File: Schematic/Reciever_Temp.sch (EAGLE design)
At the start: 5 parts, among them IC1 ATMEGA328P, IC2 LTC485N, IC3 78L05Z, IC4 LM50

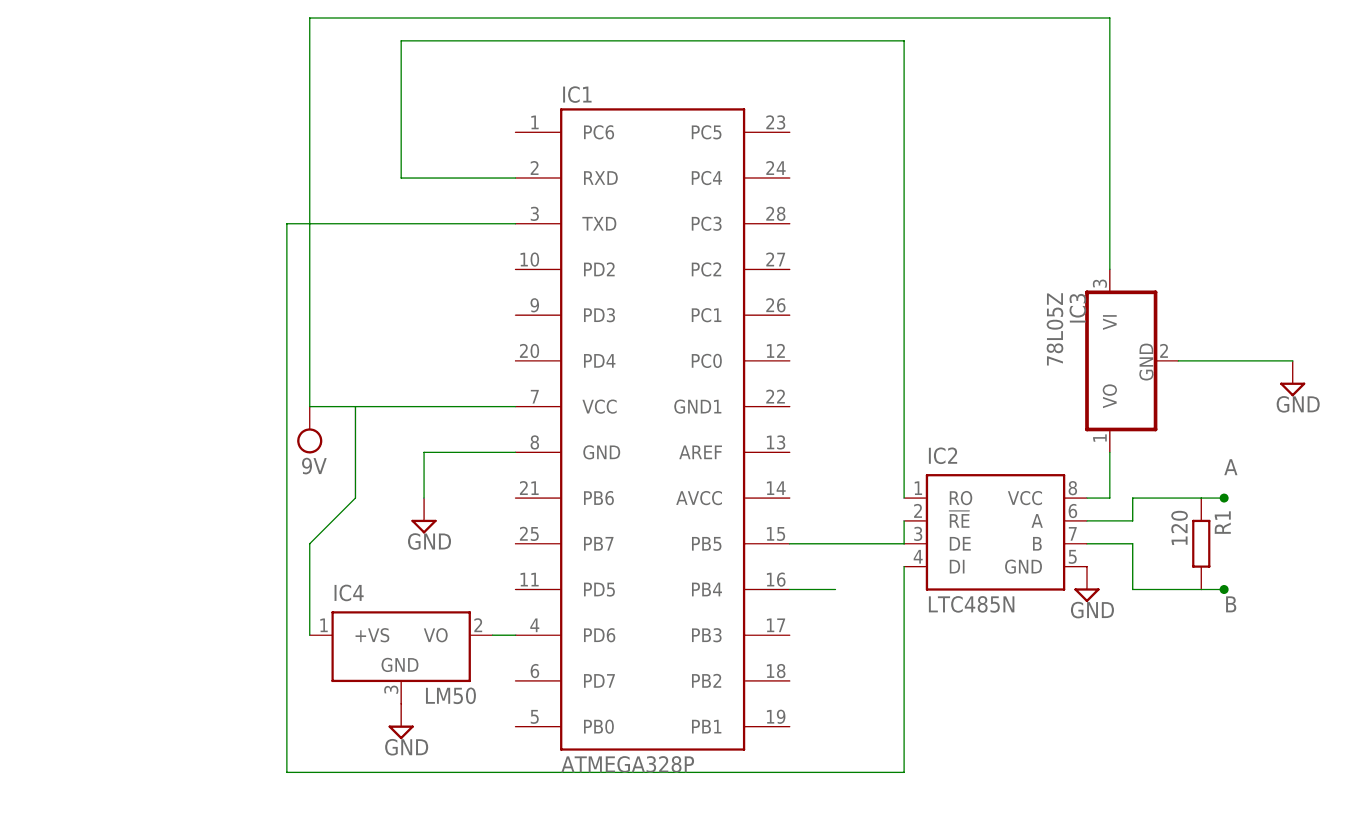
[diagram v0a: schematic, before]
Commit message: Gør klar til eksamen
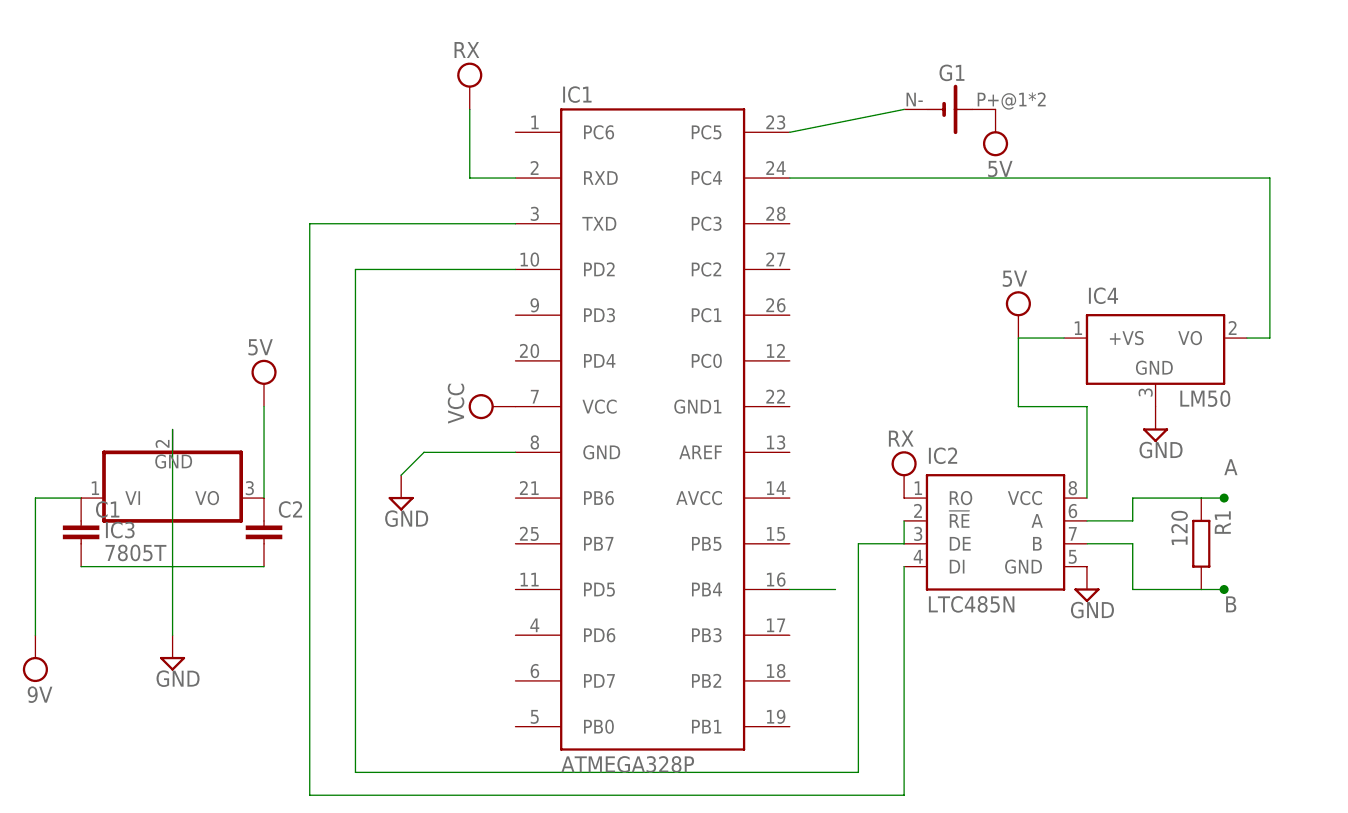
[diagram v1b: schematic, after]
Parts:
- added C1, C2: (no value), rcl:C-EU050-030X075
- added G1: BATTERY-HOLDER_11.6MM, battery:BATTERY-HOLDER_11.6MM
- IC3: value 78L05Z -> 7805T; device linear:78L05Z -> linear:7805T
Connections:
- removed net N$1: IC1.PB5, IC2.!RE, IC2.DE
- net GND: now also C1.2, C2.2
- net N$2: now also G1.-, IC1.PC5; no longer IC1.RXD, IC2.RO
- net N$4: now also IC1.PD2, IC2.!RE, IC2.DE; no longer IC2.VCC, IC3.VO
- net N$6: now also IC1.PC4; no longer IC1.PD6
- net VCC: now also C1.1, C2.1, G1.+, IC1.RXD, IC2.RO, IC2.VCC, IC3.VO
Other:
- moved on the sheet: IC3, IC4
